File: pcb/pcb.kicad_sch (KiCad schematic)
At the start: 140 parts, among them P1 L to R, P2 R to computer, P3 R to L, SW1 SW_SPST, SW10 SW_SPST, SW11 SW_SPST, SW12 SW_SPST, SW13 SW_SPST, SW14 SW_SPST, SW15 SW_SPST, SW16 SW_SPST, SW17 SW_SPST, SW18 SW_SPST, SW19 SW_SPST, SW2 SW_SPST, SW20 SW_SPST, SW21 SW_SPST, SW22 SW_SPST, SW23 SW_SPST, SW24 SW_SPST, SW25 SW_SPST, SW26 SW_SPST, SW27 SW_SPST, SW28 SW_SPST, SW29 SW_SPST, SW3 SW_SPST, SW30 SW_SPST, SW31 SW_SPST, SW32 SW_SPST, SW33 SW_SPST, SW34 SW_SPST, SW35 SW_SPST, SW36 SW_SPST, SW37 SW_SPST, SW38 SW_SPST, SW39 SW_SPST, SW4 SW_SPST, SW40 SW_SPST, SW41 SW_SPST, SW42 SW_SPST, SW43 SW_SPST, SW44 SW_SPST, SW45 SW_SPST, SW46 SW_SPST, SW47 SW_SPST, SW48 SW_SPST, SW49 SW_SPST, SW5 SW_SPST, SW50 SW_SPST, SW51 SW_SPST, SW52 SW_SPST, SW53 SW_SPST, SW54 SW_SPST, SW55 SW_SPST, SW56 SW_SPST, SW57 SW_SPST, SW58 SW_SPST, SW59 SW_SPST, SW6 SW_SPST, SW60 SW_SPST, SW61 SW_SPST, SW62 SW_SPST, SW63 SW_SPST, SW64 SW_SPST, SW7 SW_SPST, SW8 SW_SPST, SW9 SW_SPST, U1 ATmega16U4-A, U2 ATmega16U4-A

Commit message: upd and add switches submodule
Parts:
- C1, C2, C3, C4, C6: footprint (none) -> Capacitor_SMD:C_1206_3216Metric_Pad1.33x1.80mm_HandSolder
- P1: footprint (none) -> Connector_USB:USB_C_Plug_JAE_DX07P024AJ1
- P2, P3: footprint (none) -> Connector_USB:USB_C_Plug_Molex_105444
- R3, R4, R6: footprint (none) -> Resistor_SMD:R_1206_3216Metric_Pad1.30x1.75mm_HandSolder
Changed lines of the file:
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@@
 			)
 		)
-		(property "Footprint" ""
+		(property "Footprint" "Resistor_SMD:R_1206_3216Metric_Pad1.30x1.75mm_HandSolder"
 			(at 355.6 166.878 90)
 			(show_name yes)
@@
 			)
 		)
-		(property "Footprint" ""
+		(property "Footprint" "Capacitor_SMD:C_1206_3216Metric_Pad1.33x1.80mm_HandSolder"
 			(at 390.8552 96.52 0)
 			(effects
@@
 			)
 		)
-		(property "Footprint" ""
+		(property "Footprint" "Connector_USB:USB_C_Plug_Molex_105444"
 			(at 300.99 176.53 0)
 			(effects
@@
 			)
 		)
-		(property "Footprint" ""
+		(property "Footprint" "Capacitor_SMD:C_1206_3216Metric_Pad1.33x1.80mm_HandSolder"
 			(at 390.8552 187.96 0)
 			(effects
@@
 			)
 		)
-		(property "Footprint" ""
+		(property "Footprint" "Capacitor_SMD:C_1206_3216Metric_Pad1.33x1.80mm_HandSolder"
 			(at 375.6152 161.29 0)
 			(effects
@@
 			)
 		)
-		(property "Footprint" ""
+		(property "Footprint" "Capacitor_SMD:C_1206_3216Metric_Pad1.33x1.80mm_HandSolder"
 			(at 375.6152 187.96 0)
 			(effects
@@
 			)
 		)
-		(property "Footprint" ""
+		(property "Footprint" "Resistor_SMD:R_1206_3216Metric_Pad1.30x1.75mm_HandSolder"
 			(at 355.6 179.578 90)
 			(effects
@@
 			)
 		)
-		(property "Footprint" ""
+		(property "Footprint" "Capacitor_SMD:C_1206_3216Metric_Pad1.33x1.80mm_HandSolder"
 			(at 390.8552 161.29 0)
 			(effects
@@
 			)
 		)
-		(property "Footprint" ""
+		(property "Footprint" "Connector_USB:USB_C_Plug_JAE_DX07P024AJ1"
 			(at 261.62 176.53 0)
 			(effects
@@
 			)
 		)
-		(property "Footprint" ""
+		(property "Footprint" "Resistor_SMD:R_1206_3216Metric_Pad1.30x1.75mm_HandSolder"
 			(at 355.6 174.498 90)
 			(effects
@@
 			)
 		)
-		(property "Footprint" ""
+		(property "Footprint" "Connector_USB:USB_C_Plug_Molex_105444"
 			(at 340.36 175.26 0)
 			(effects

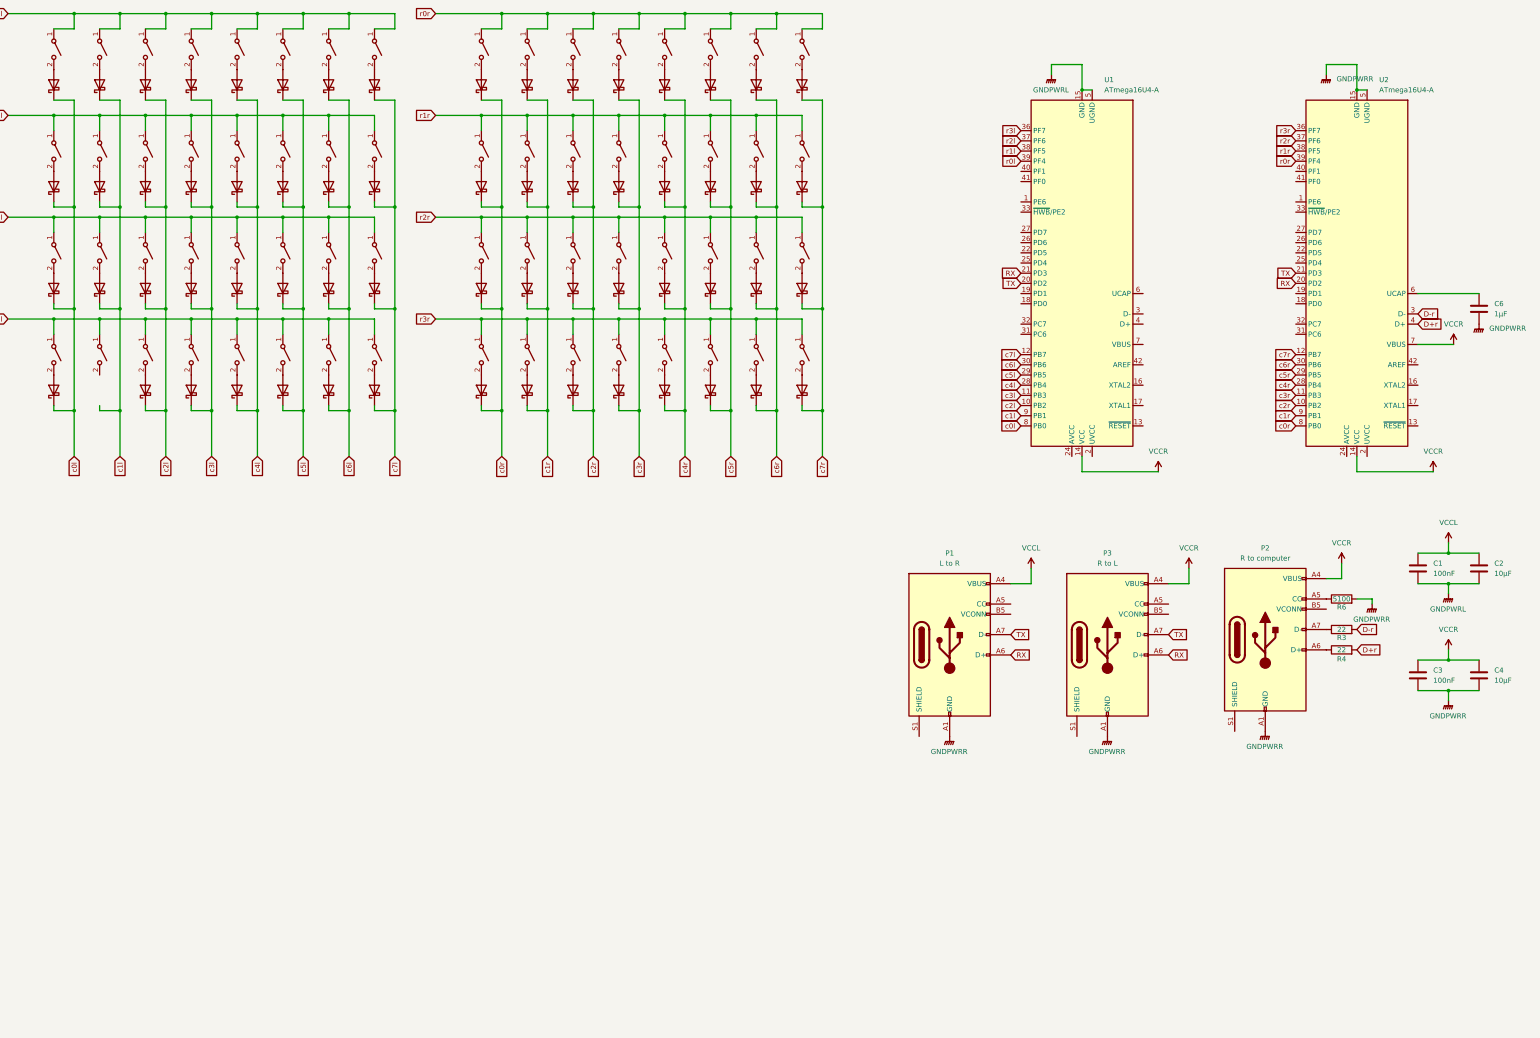
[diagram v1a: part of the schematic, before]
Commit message: upd
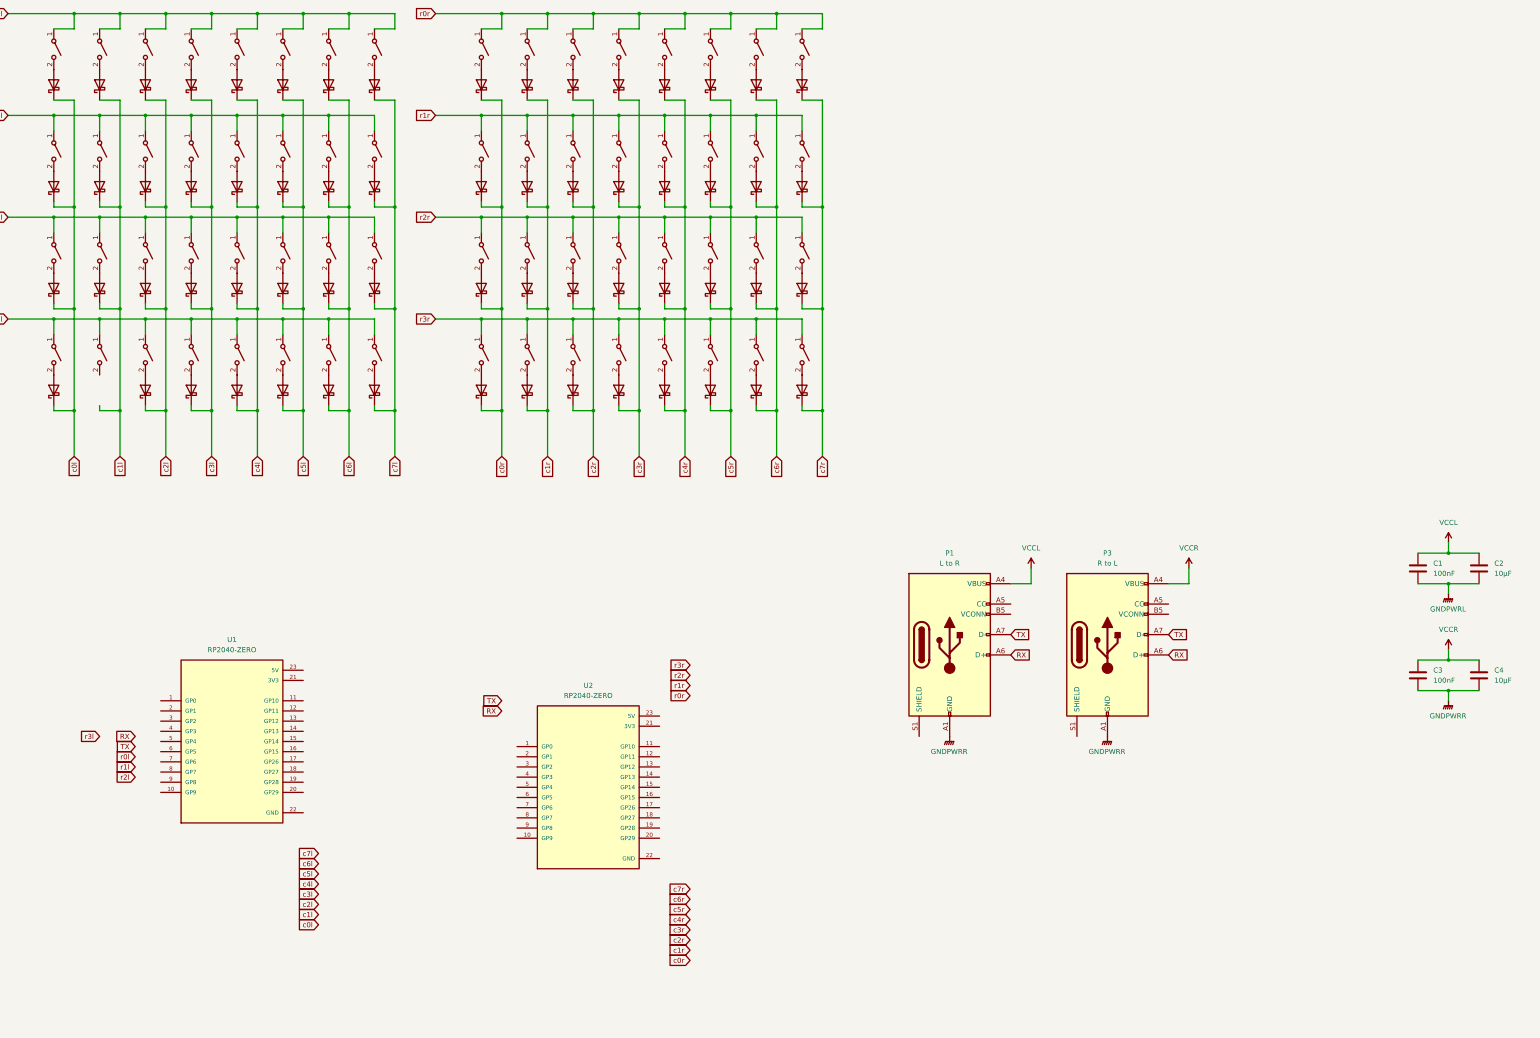
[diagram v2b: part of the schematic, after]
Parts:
- removed C6: 1µF, Capacitor_SMD:C_1206_3216Metric_Pad1.33x1.80mm_HandSolder, symbol Device:C
- removed P2: R to computer, Connector_USB:USB_C_Plug_Molex_105444, symbol Connector:USB_C_Plug_USB2.0
- removed R3, R4: 22, Resistor_SMD:R_1206_3216Metric_Pad1.30x1.75mm_HandSolder, symbol Device:R
- removed R6: 5100, Resistor_SMD:R_1206_3216Metric_Pad1.30x1.75mm_HandSolder, symbol Device:R
- removed U1, U2: ATmega16U4-A, Package_QFP:TQFP-44_10x10mm_P0.8mm, symbol MCU_Microchip_ATmega:ATmega16U4-A
- added U1, U2: RP2040-ZERO, RP2040-ZERO:MODULE_RP2040-ZERO, symbol RP2040:RP2040-ZERO
- SW1, SW10, SW11, SW12, SW13, SW14, SW15, SW16, SW17, SW18, SW19, SW2, SW20, SW21, SW22, SW23, SW24, SW25, SW26, SW27, SW28, SW29, SW3, SW30, SW31, SW32, SW33, SW34, SW35, SW36, SW37, SW38, SW39, SW4, SW40, SW41, SW42, SW43, SW44, SW45, SW46, SW47, SW48, SW49, SW5, SW50, SW51, SW52, SW53, SW54, SW55, SW56, SW57, SW58, SW59, SW6, SW60, SW61, SW62, SW63, SW64, SW7, SW8, SW9: footprint (none) -> Footprints:SW_MX_THT
